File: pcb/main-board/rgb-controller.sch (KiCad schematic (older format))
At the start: 23 parts, among them IC1 ATMEGA328-P, J1 LCD_HEADER, J2 CONTROL_HEADER, J3 UART_HEADER, J4 LED_HEADER, J5 PWR_IN, Q1 STP35NF10, Q2 STP35NF10, Q3 STP35NF10, SW1 SW_PUSH, SW2 SW_POWER, U1 7805_NUM, X1 16MHz

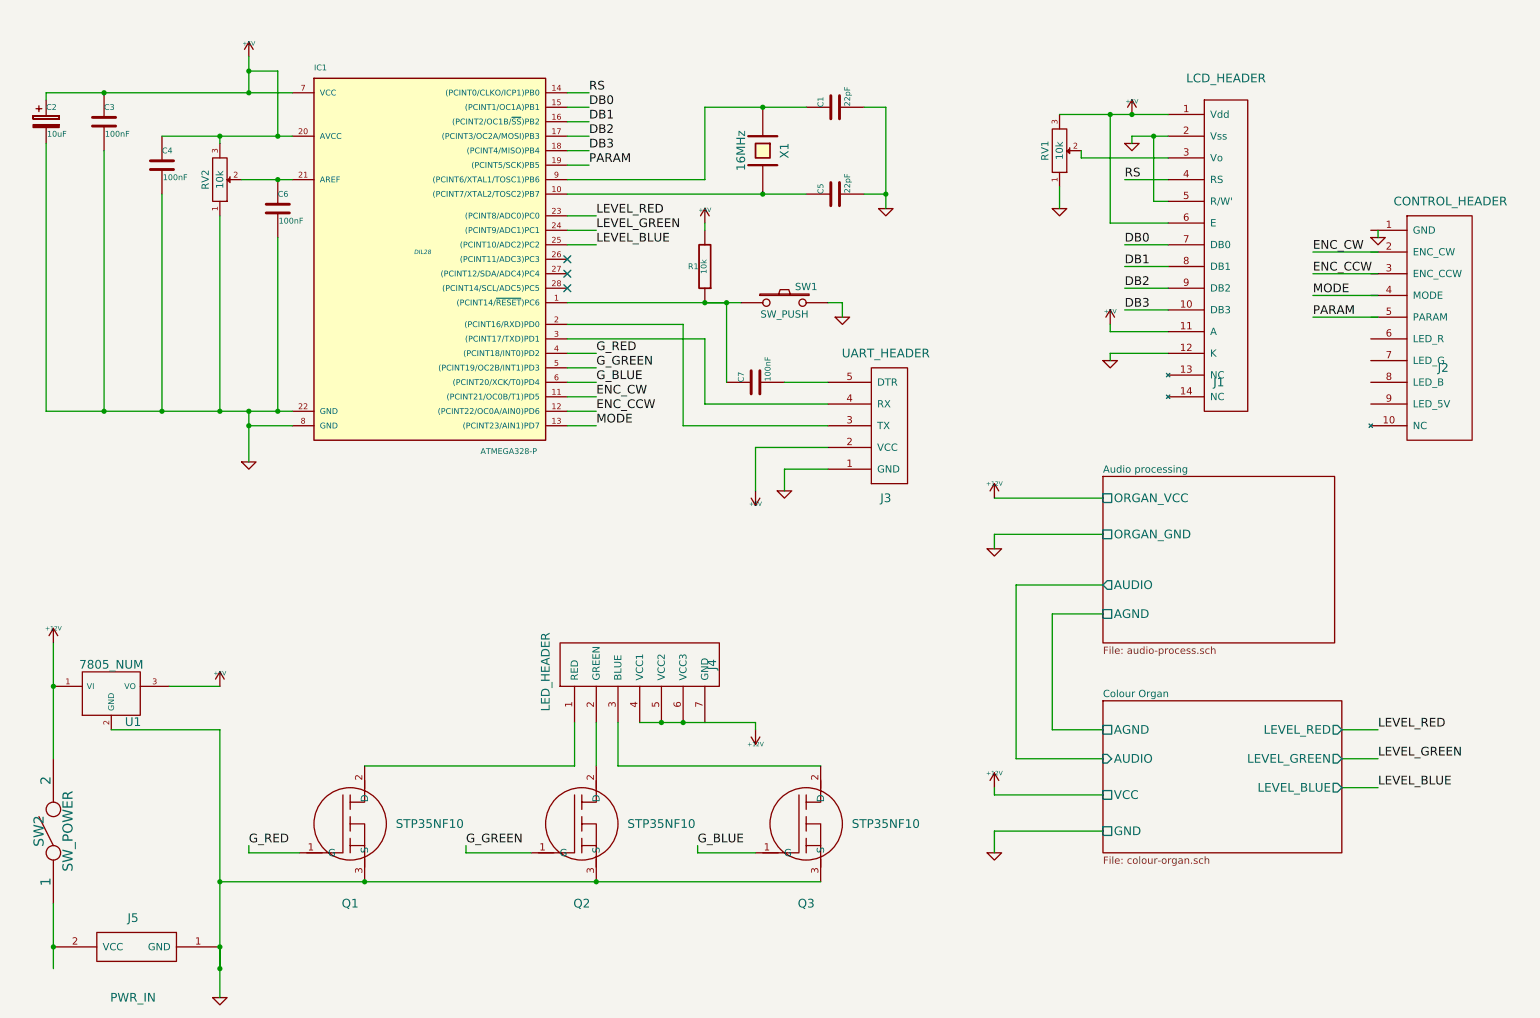
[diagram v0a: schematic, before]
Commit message: working on finding components for parts
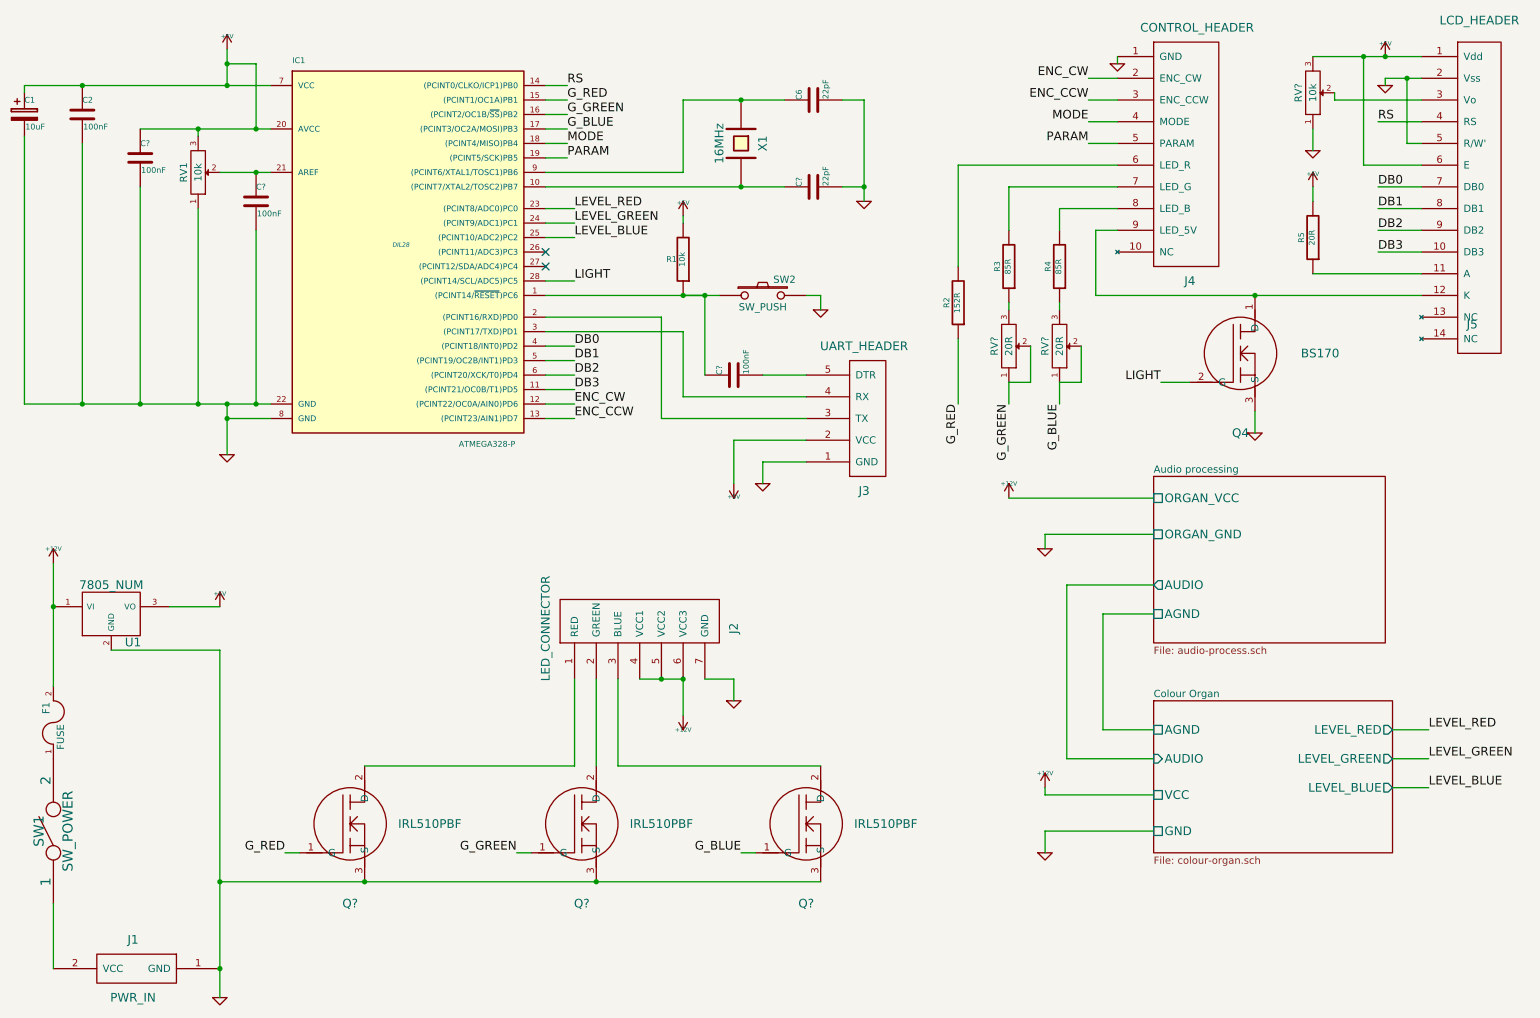
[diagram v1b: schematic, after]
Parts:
- removed C4, C6, C7: 100nF, ~, symbol C-rgb
- removed C5: 22pF, ~, symbol C-RESCUE-rgb-controller
- removed J2: CONTROL_HEADER, symbol CONTROL_HEADER
- removed J5: PWR_IN, ~, symbol PWR_IN
- removed Q1, Q2, Q3: STP35NF10, symbol STP35NF10
- removed RV1: 10k, ~, symbol POT-rgb
- added C? (x3): 100nF, ~, symbol C-rgb
- added C?: 22pF, ~, symbol C-RESCUE-rgb-controller
- added F1: FUSE, symbol FUSE
- added J1: PWR_IN, symbol PWR_IN
- added J4: CONTROL_HEADER, symbol CONTROL_HEADER
- added Q4: BS170, symbol BS170
- added Q? (x3): IRL510PBF, symbol IRL510PBF
- added R2: 152R, symbol R-rgb
- added R3, R4: 85R, symbol R-rgb
- added R5: 20R, symbol R-rgb
- added RV? (x2): 20R, ~, symbol POT-rgb
- added RV?: 10k, ~, symbol POT-rgb
- C1: renamed from C2; Manufacturer Vishay -> Kemet; Order (none) -> No; Product code 489D106X0016C1VE3 -> T350E106M025AT; Product description Tantalum Capacitor, Resin Coated, 489D Series, 10 µF, ± 20%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 -> 10µF Conformal Coated Tantalum Capacitors 25V Radial 2.5 Oh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; Supplier Farnell -> Digikey; Supplier URL (none) -> http://www.digikey.co.uk/product-detail/en/kemet/T350E106M0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; Supplier code 1753975 -> 399-9907-ND
- C2: renamed from C3; Manufacturer Multicomp -> Kemet; Order (none) -> No; Product code MC0805Y104M500A2.54MM -> C315C104M5U5TA; Product description Multilayer Ceramic Capacitor, MC Series, 0.1 µF, ± 20%, Y5V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 -> 0.10µF 50V Ceramic Capacitor Z5U Radial 0.150\" L x 0.100\"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; Supplier Farnell -> Digikey; Supplier URL (none) -> http://www.digikey.co.uk/product-detail/en/kemet/C315C104M5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; Supplier code 2112751 -> 399-4151-ND
- C6: renamed from C1; Manufacturer (none) -> Kemet; Order (none) -> No; Product code (none) -> C315C220J5G5TA; Product description (none) -> 22pF 50V Ceramic Capacitor C0G, NP0 Radial 0.150\" L x 0.10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; Supplier Have -> Digikey; Supplier URL (none) -> http://www.digikey.co.uk/product-detail/en/kemet/C315C220J5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; Supplier code (none) -> 399-9721-ND
- IC1: Manufacturer Atmel -> Arduino; Order (none) -> No; Product code AT-MEGA328-P -> A000048; Supplier Have -> Digikey; Supplier URL (none) -> http://www.digikey.co.uk/product-search/en/integrated-circu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; Supplier code (none) -> 1050-1019-ND
- J2: renamed from J4; value LED_HEADER -> LED_CONNECTOR; Manufacturer (none) -> CUI Inc.; Notes (none) -> Rated to 2A per conductor at 12V DC; Order (none) -> No; Product code (none) -> MD-60S; Product description (none) -> 6 Position Circular Connector Receptacle, Female Sockets So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; Supplier (none) -> Digikey; Supplier URL (none) -> http://www.digikey.co.uk/product-detail/en/cui-inc/MD-60S/C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; Supplier code (none) -> CP-2460-ND
- R1: Manufacturer (none) -> Stackpole Electronics Inc.; Order (none) -> No; Product code (none) -> CF18JT10K0; Product description (none) -> RES 10K OHM 1/8W 5% CF AXIAL; Supplier (none) -> Digikey; Supplier URL (none) -> http://www.digikey.co.uk/product-detail/en/stackpole-electr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; Supplier code (none) -> CF18JT10K0CT-ND
- RV1: renamed from RV2; Manufacturer (none) -> Bourns Inc.; Order (none) -> No; Product code (none) -> 3362P-1-103LF; Product description (none) -> 10k Ohm 0.5W, 1/2W PC Pins Through Hole Trimmer Potentiomet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; Supplier (none) -> Digikey; Supplier URL (none) -> http://www.digikey.co.uk/product-detail/en/bourns-inc/3362P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; Supplier code (none) -> 3362P-103LF-ND
- SW1: renamed from SW2; Manufacturer (none) -> C&K Components; Order (none) -> No; Product code (none) -> E101J1AQE2; Product description (none) -> Rocker Switch SPDT 7.5A (AC/DC) 125V Through Hole, Right An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; Supplier (none) -> Digikey; Supplier URL (none) -> http://www.digikey.co.uk/product-detail/en/c-k-components/E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; Supplier code (none) -> CKN2070-ND
- U1: Manufacturer (none) -> ON Semiconductor; Order (none) -> No; Product code (none) -> NCP7805TG; Product description (none) -> Linear Voltage Regulator IC Positive Fixed 1 Output 5V 1A T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; Supplier (none) -> Digikey; Supplier URL (none) -> http://www.digikey.co.uk/product-detail/en/on-semiconductor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; Supplier code (none) -> NCP7805TGOS-ND
- renumbered J1 to J5, SW1 to SW2
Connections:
- net labels added: LIGHT
- wire segments 115 -> 159
- no-connect marks 3 -> 2
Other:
- moved on the sheet: C1, C2, C6, IC1, J2, J3, J5, R1, RV1, SW2, U1, X1
